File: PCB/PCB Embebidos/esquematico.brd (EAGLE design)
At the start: 91 x 70.9 mm, 30 parts, among them IC1 LM358N, IC2 317T, T1 BT138-V

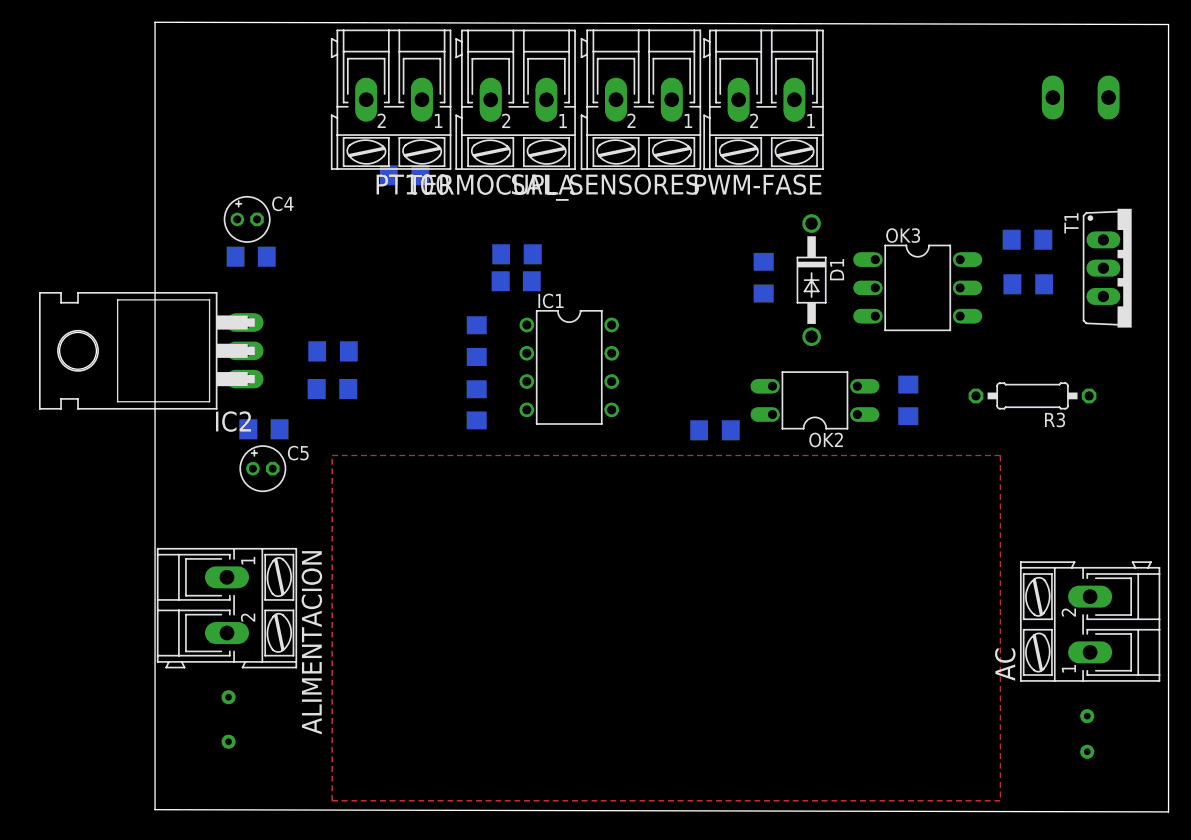
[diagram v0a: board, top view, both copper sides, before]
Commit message: Estuve ruteando el PCB. Creo que esta terminado, pero tendria que revisarlo menos dormido
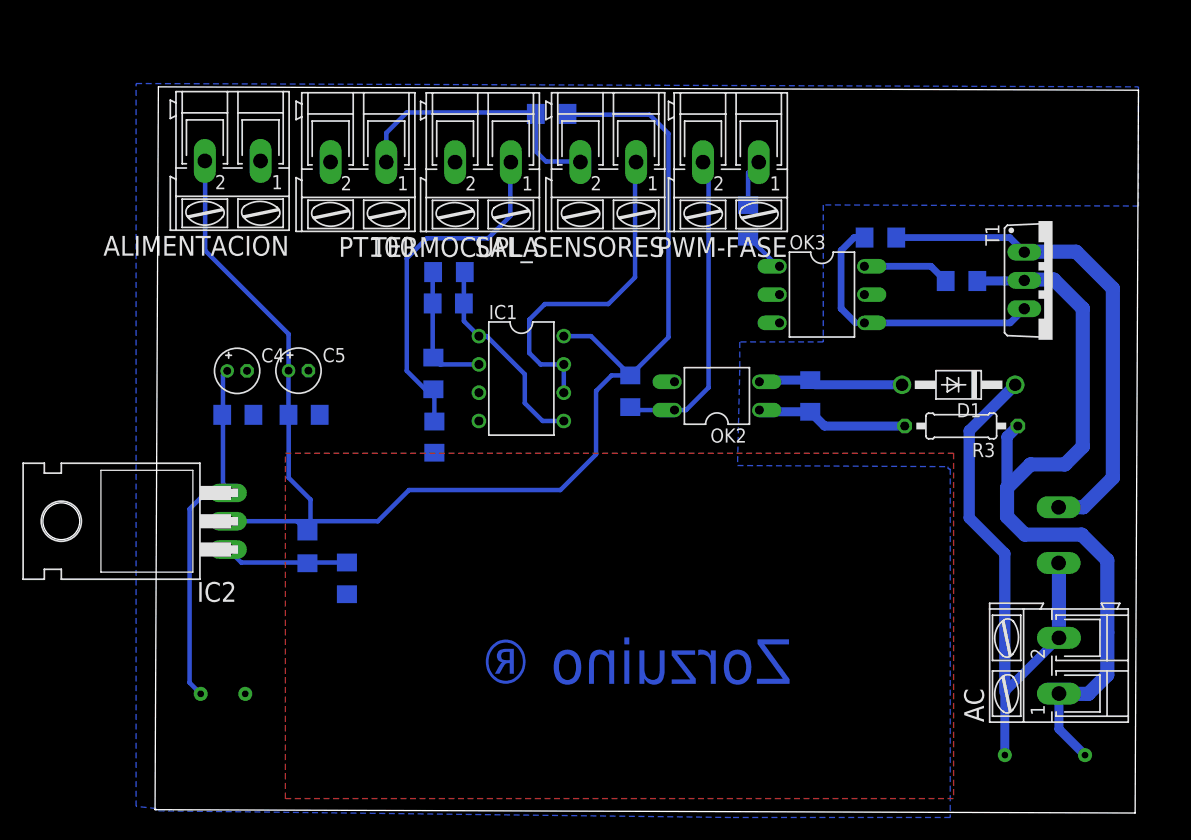
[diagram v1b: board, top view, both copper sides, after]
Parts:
- moved ALIMENTACION 39.9 mm to (6.96, 58.2), turned to 180 degrees
- moved CARGA 39.4 mm to (81.1, 24.6), turned to 270 degrees
- moved R9 17.7 mm to (13.7, 23.6), turned to 270 degrees
- moved R11 17.0 mm to (17.2, 20.8), turned to 270 degrees
- moved D1 16.2 mm to (72.2, 38.1), turned to 180 degrees
- moved IC2 15.4 mm to (-3.59, 25.9)
- moved R10 14.3 mm to (35.6, 62.5), turned to 0 degrees
- moved C1 14.3 mm to (7.43, 35.5)
- moved C4 13.6 mm to (7.37, 39.4)
- moved R2 13.2 mm to (65.1, 51.4)
- moved C5 9.36 mm to (12.9, 39.4)
- moved OK2 8.81 mm to (50.5, 37.1)
- moved R6 8.81 mm to (58.8, 37.1)
- moved OK3 8.62 mm to (59.9, 46.2)
- moved R5 8.37 mm to (42.7, 37.6), turned to 90 degrees
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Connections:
- net AC-: now also AC.2, CARGA.2; no longer CARGA.1
- net GND: now also ALIMENTACION.1, OK3.2; no longer ALIMENTACION.2
- net N$4: now also CARGA.1; no longer CARGA.2
- net VCC: now also ALIMENTACION.2; no longer ALIMENTACION.1
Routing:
- net VCC: track 0.00 -> 125.6 mm
- net AC+: track 0.00 -> 72.6 mm
- net AC-: track 0.00 -> 49.9 mm
- net N$4: track 0.00 -> 44.3 mm
- net VCC_5V: track 0.00 -> 32.6 mm
- net TERMOCUPLA: track 0.00 -> 31.8 mm
- net SAL_TERMOCUPLA: track 0.00 -> 30.6 mm
- net FASE: track 0.00 -> 28.4 mm
- net SAL_PT100: track 0.00 -> 25.6 mm
- net N$8: track 0.00 -> 25.3 mm
- net N$7: track 0.00 -> 18.6 mm
- net N$3: track 0.00 -> 13.6 mm
- net N$9: track 0.00 -> 13.0 mm
- net N$5: track 0.00 -> 12.1 mm
- net N$6: track 0.00 -> 11.9 mm
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- added copper zone on layer 16, net GND
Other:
- board size 91 x 70.9 mm -> 88.3 x 65.2 mm
- board text added: "Zorzuino ®"
